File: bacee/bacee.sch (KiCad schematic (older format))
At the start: 13 parts, among them U1 24LC1025, U2 24LC1025, U3 DS13375+, U4 ATMEGA328P-AU, Y1 Crystal 32MHz, Y2 Crystal 16MHz

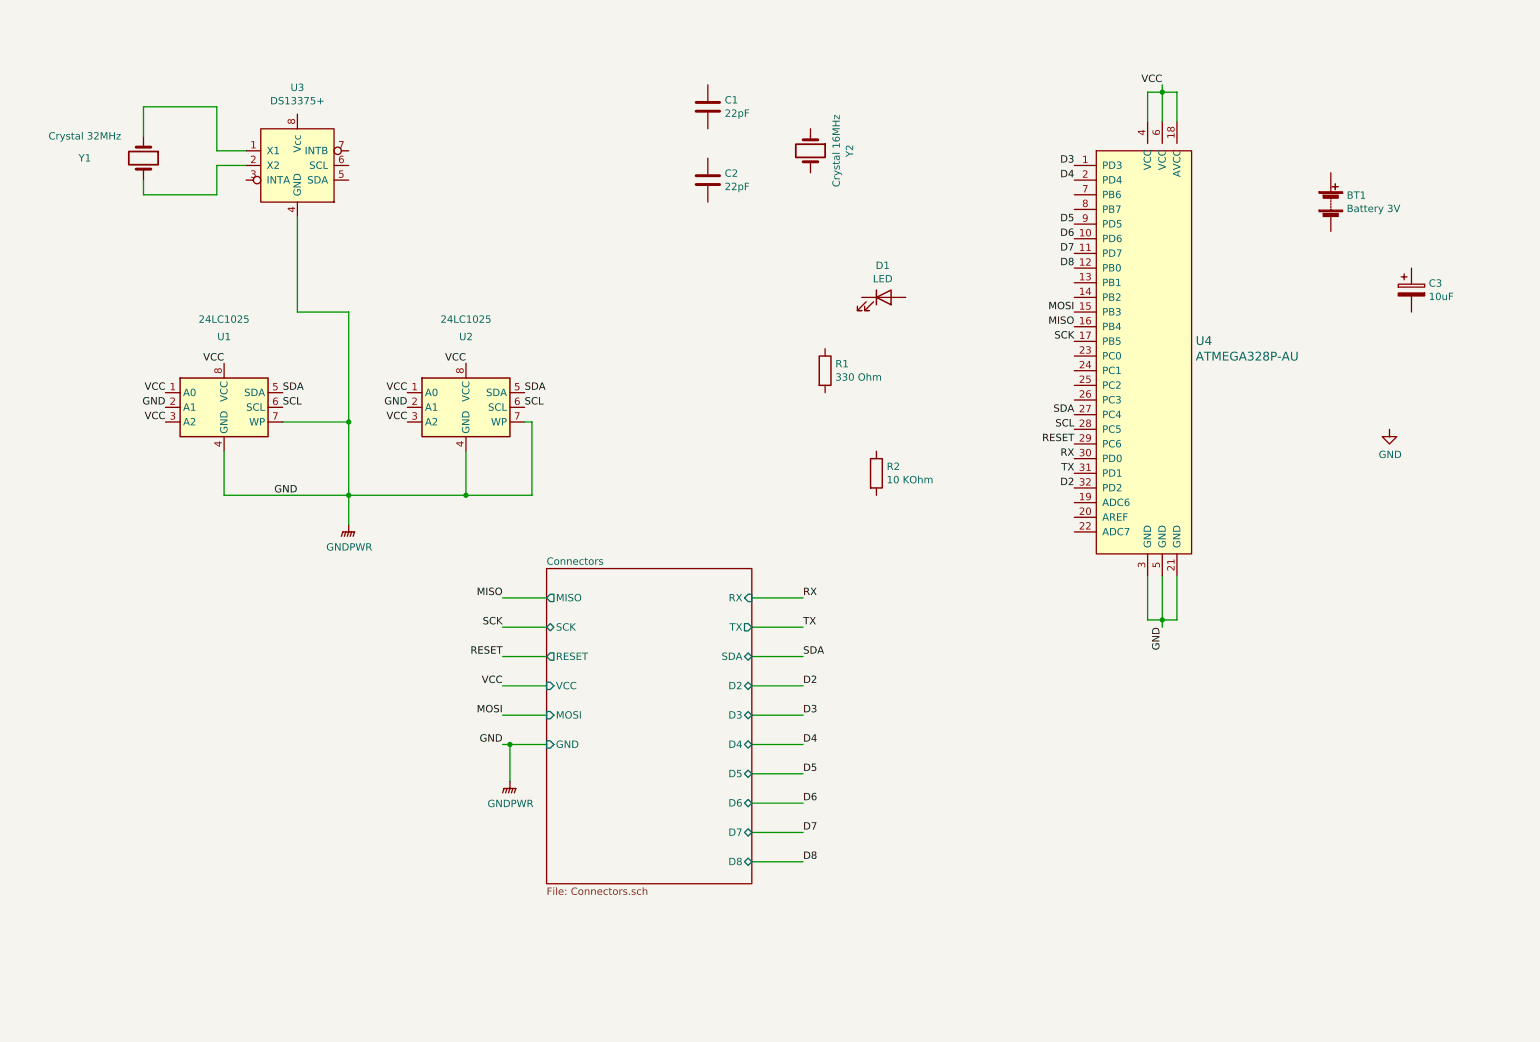
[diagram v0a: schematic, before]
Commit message: done
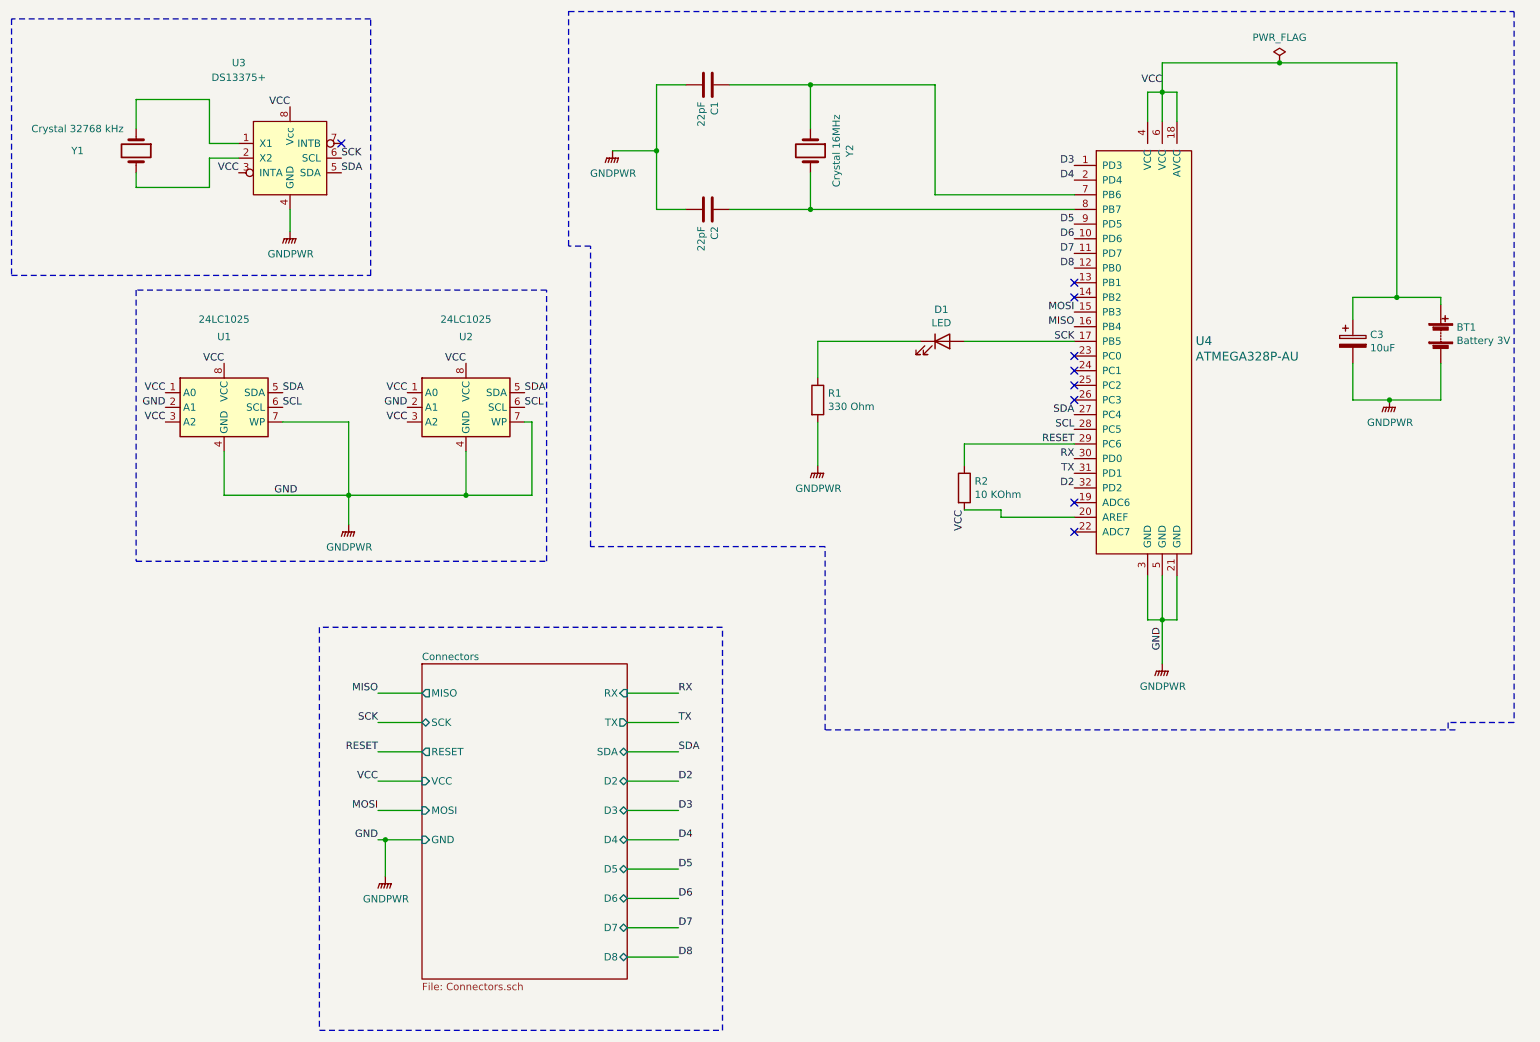
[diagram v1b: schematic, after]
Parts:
- Y1: value Crystal 32MHz -> Crystal 32768 kHz
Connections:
- net GND is gone; now on net GNDPWR: U1.2 (A1), U1.4 (GND), U1.7 (WP), U2.2 (A1), U2.4 (GND), U2.7 (WP), U3.4 (GND), U4.21 (GND), U4.3 (GND), U4.5 (GND)
- net RESET: now also R2.1
- net SCK: now also D1.2 (A), U3.6 (SCL)
- net SDA: now also U3.5 (SDA)
- net VCC: now also BT1.1 (+), C3.1, R2.2, U3.3 (INTA), U3.8 (Vcc), U4.20 (AREF)
- net GNDPWR: now reaches BT1.2 (-)
- net GNDPWR: now also C1.2, C2.2, C3.2, R1.2
- net at C1.1: now also U4.7 (PB6), Y2.1
- net at C2.1: now also U4.8 (PB7), Y2.2
- net at D1.1 (K): now also R1.1
- no-connect marks 0 -> 9
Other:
- moved on the sheet: BT1, C1, C2, C3, D1, R1, R2, U3, Y1
